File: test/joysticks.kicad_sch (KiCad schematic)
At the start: 20 parts, among them J3 Conn_02x06_Odd_Even, J4 Conn_02x06_Odd_Even, J5 Conn_02x06_Odd_Even, Q13 BC848, Q15 BC848, Q16 BC808, Q17 BC808

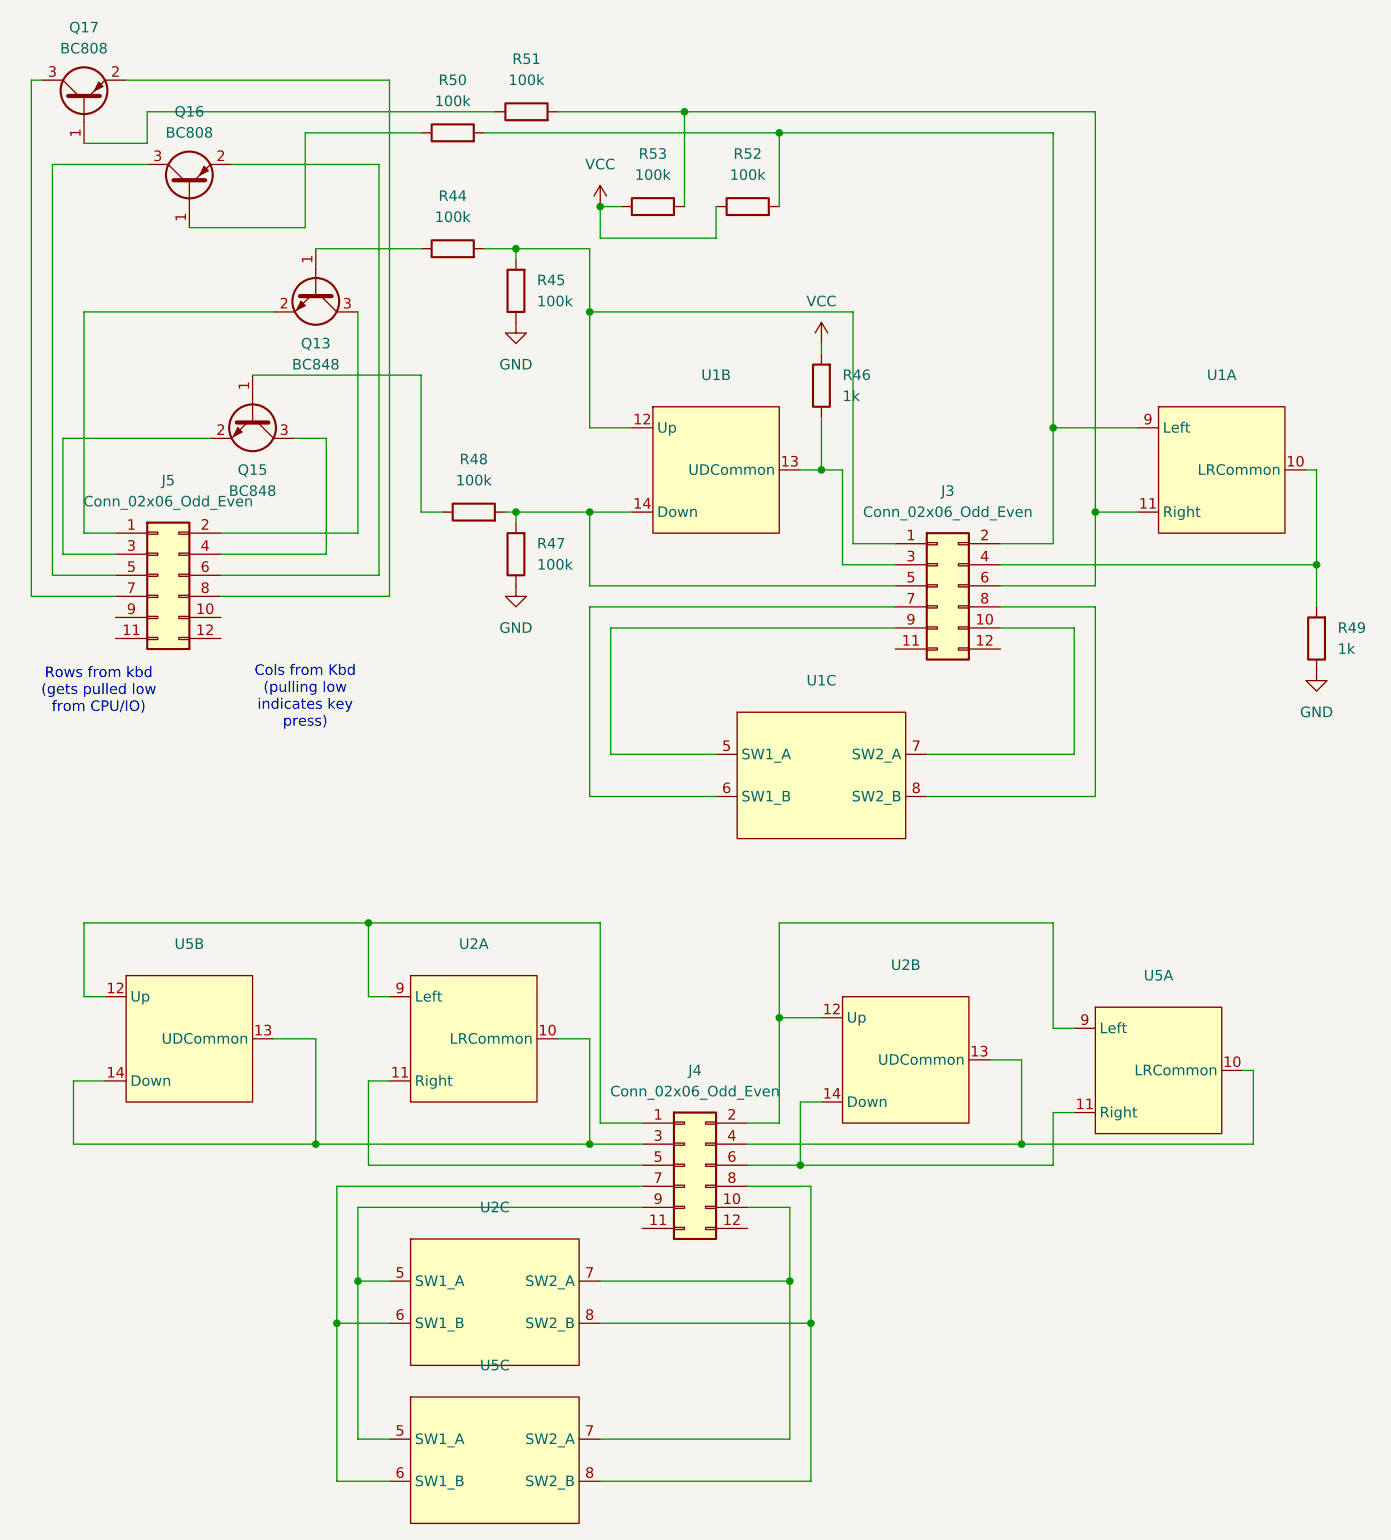
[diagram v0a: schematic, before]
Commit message: work on 2nd update test
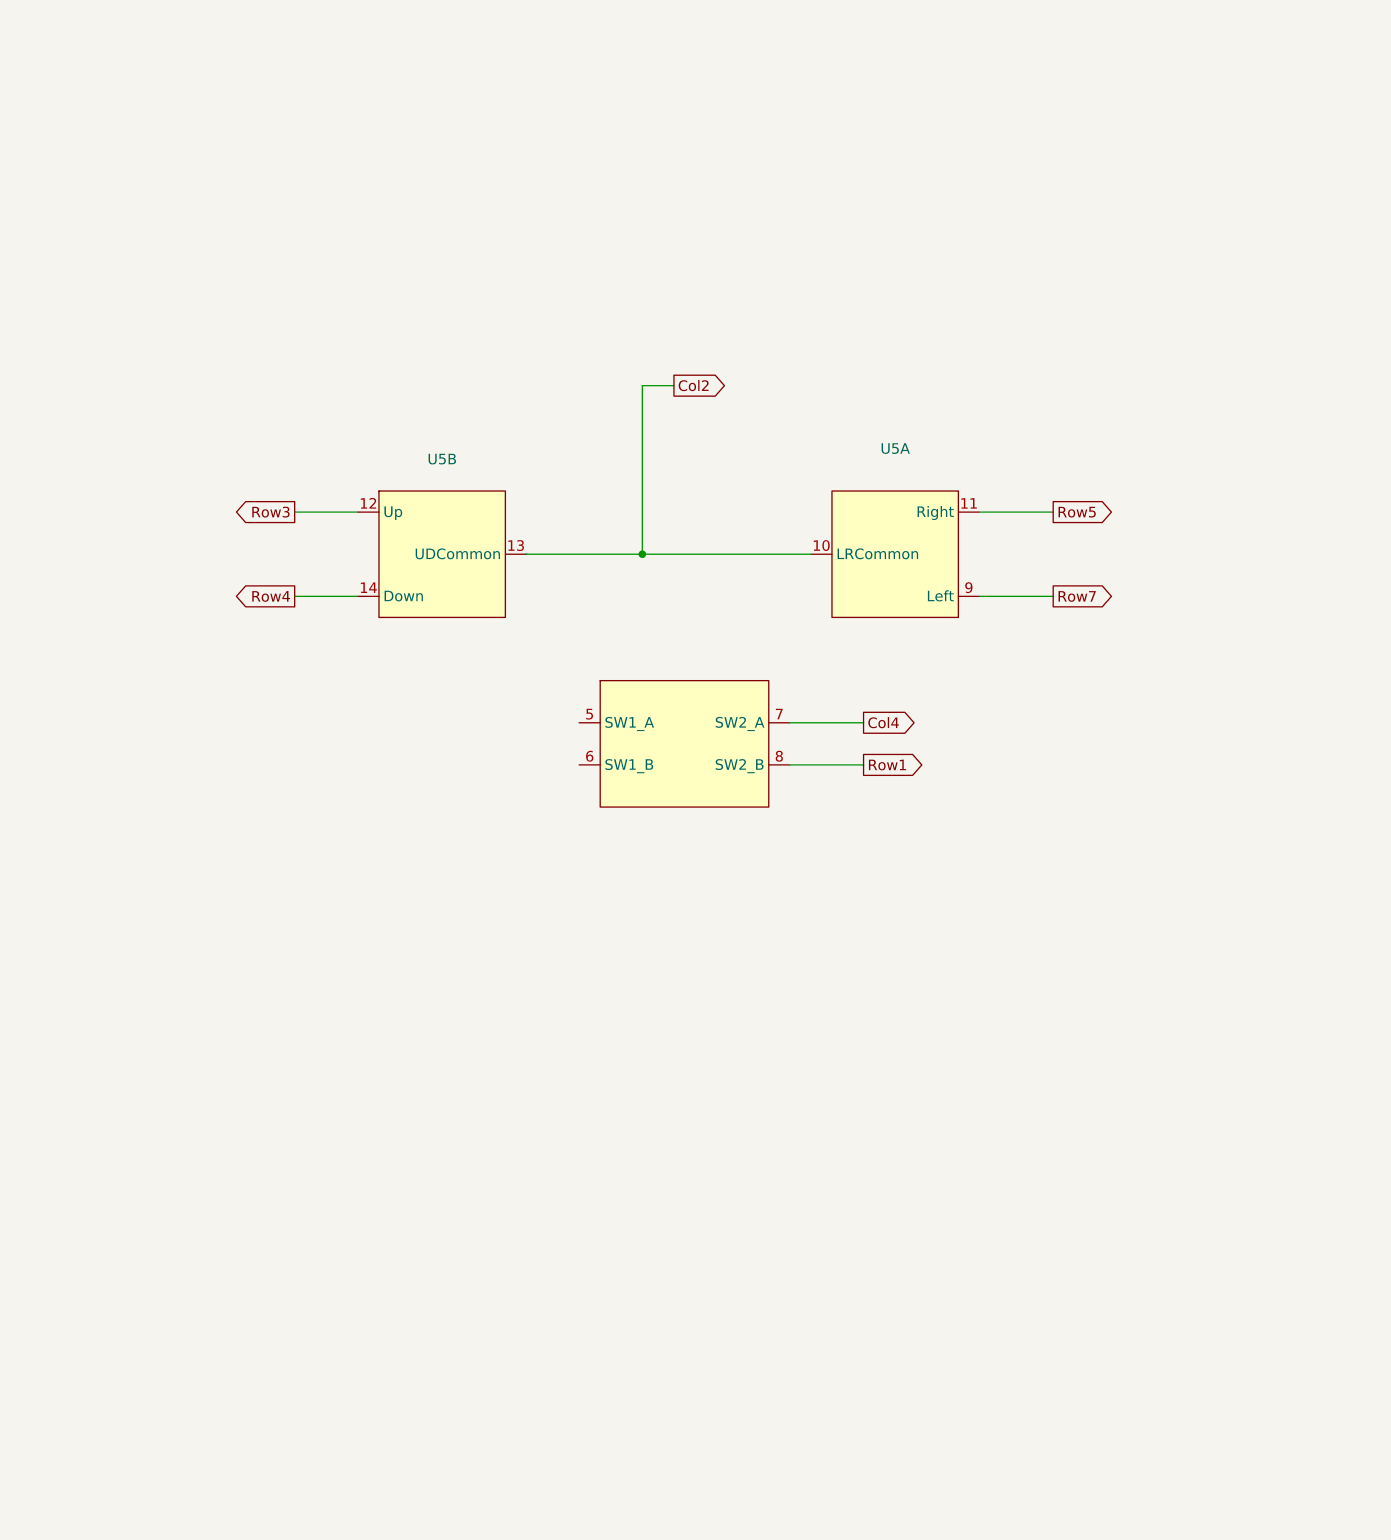
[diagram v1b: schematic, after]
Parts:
- removed J3, J4, J5: Conn_02x06_Odd_Even, Connector_PinHeader_2.54mm:PinHeader_2x06_P2.54mm_Vertical, symbol Connector_Generic:Conn_02x06_Odd_Even
- removed Q13, Q15: BC848, Package_TO_SOT_SMD:SOT-23, symbol Transistor_BJT:BC848
- removed Q16, Q17: BC808, Package_TO_SOT_SMD:SOT-23, symbol Transistor_BJT:BC808
- removed R44, R45, R47, R48, R50, R51, R52, R53: 100k, Resistor_THT:R_Axial_DIN0204_L3.6mm_D1.6mm_P2.54mm_Vertical, symbol Device:R
- removed R46, R49: 1k, Resistor_THT:R_Axial_DIN0204_L3.6mm_D1.6mm_P2.54mm_Vertical, symbol Device:R
- removed U1: ~, petkn:THB Miniature Thumbstick THB001P, symbol petkn:Thumbstick_with_switch
- removed U2: ~, petkn:true-components-98002c3-ps2-ps3, symbol petkn:Thumbstick_with_switch
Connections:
- net Col4: now reaches U5.7 (SW2_A)
- net Row1: now reaches U5.8 (SW2_B)
- net Col2: now reaches U5.10 (LRCommon)
- net Col2: now also U5.13 (UDCommon)
- net Row5: now reaches U5.11 (Right)
- net Row7: now reaches U5.9 (Left)
- net Row4: now reaches U5.14 (Down)
- net Row4: no longer U5.13 (UDCommon)
- net Row3: now reaches U5.12 (Up)
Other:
- note removed: "Cols from Kbd (pulling low indicates key press)"
- note removed: "Rows from kbd (gets pulled low from CPU/IO)"
- moved on the sheet: U5A, U5B
